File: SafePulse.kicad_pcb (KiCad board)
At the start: 4 copper layers, 40.6 x 20.8 mm, 88 parts, among them IC1 S-35770E01I-K8T2U, J1 Conn_01x03_Male, J2 4208, Q1 FQT7N10L, Q2 BC846A, Q3 MMBT3906, Q4 MMBT3906, U1 TS4061AICT-1.25, U2 74HC14, U3 TLV27L1DBVT, U33 MAX9910EXK+T, U4 CD14538BM

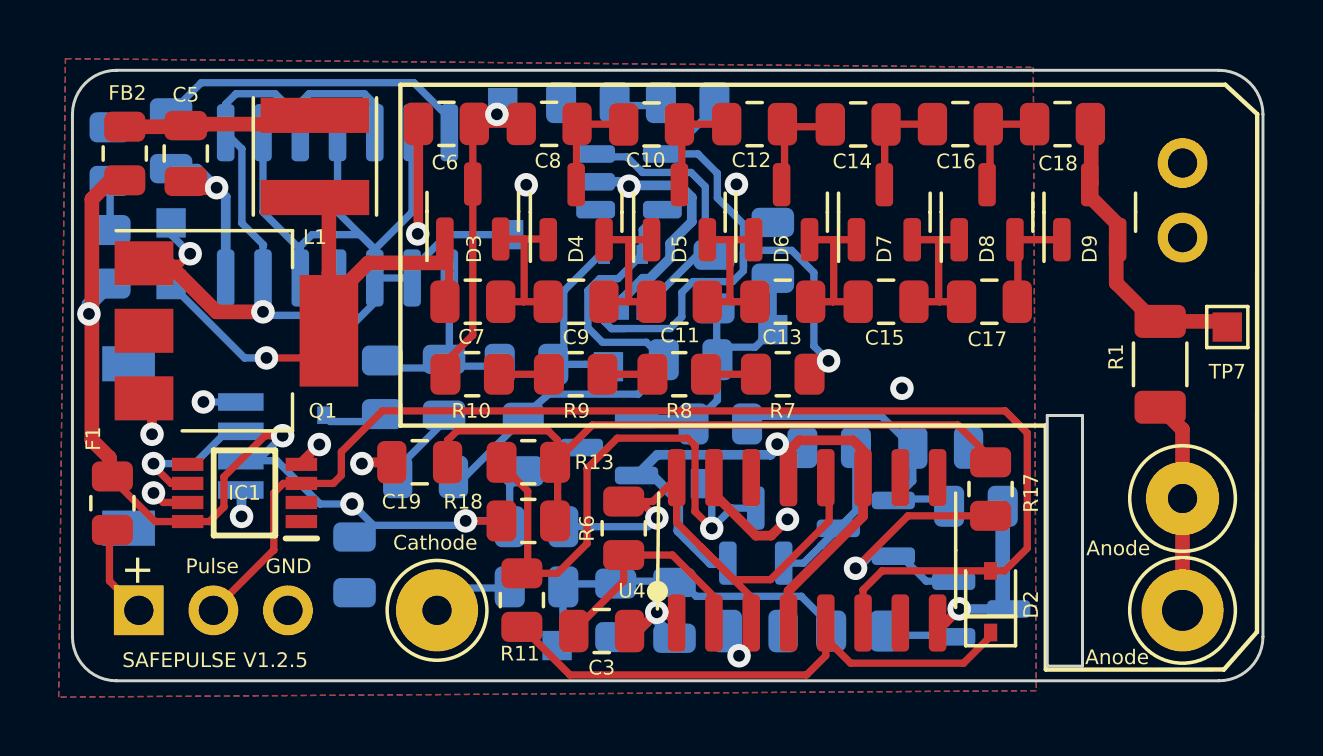
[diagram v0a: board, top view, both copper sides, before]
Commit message: Updated V1.2.4 board with new JCLPCB number
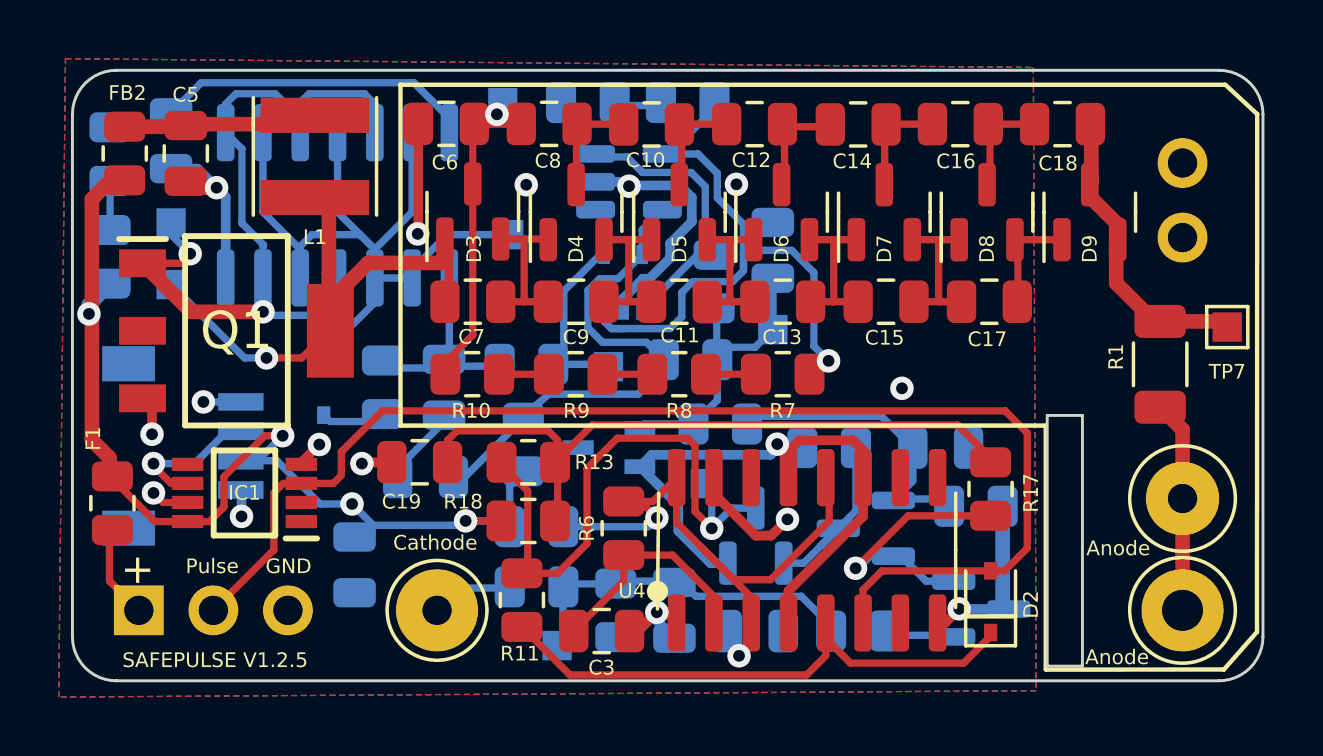
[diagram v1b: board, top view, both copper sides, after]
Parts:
- Q1: footprint Package_TO_SOT_SMD:SOT-223-3_TabPin4 -> Library:SOT230P700X180-4N
- U1: footprint Package_TO_SOT_SMD:SOT-23 -> Library:SOT65P210X110-3N
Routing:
- net GND: track 64.3 -> 63.6 mm
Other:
- copper layers 4 -> 13

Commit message: V1.2.5 boards
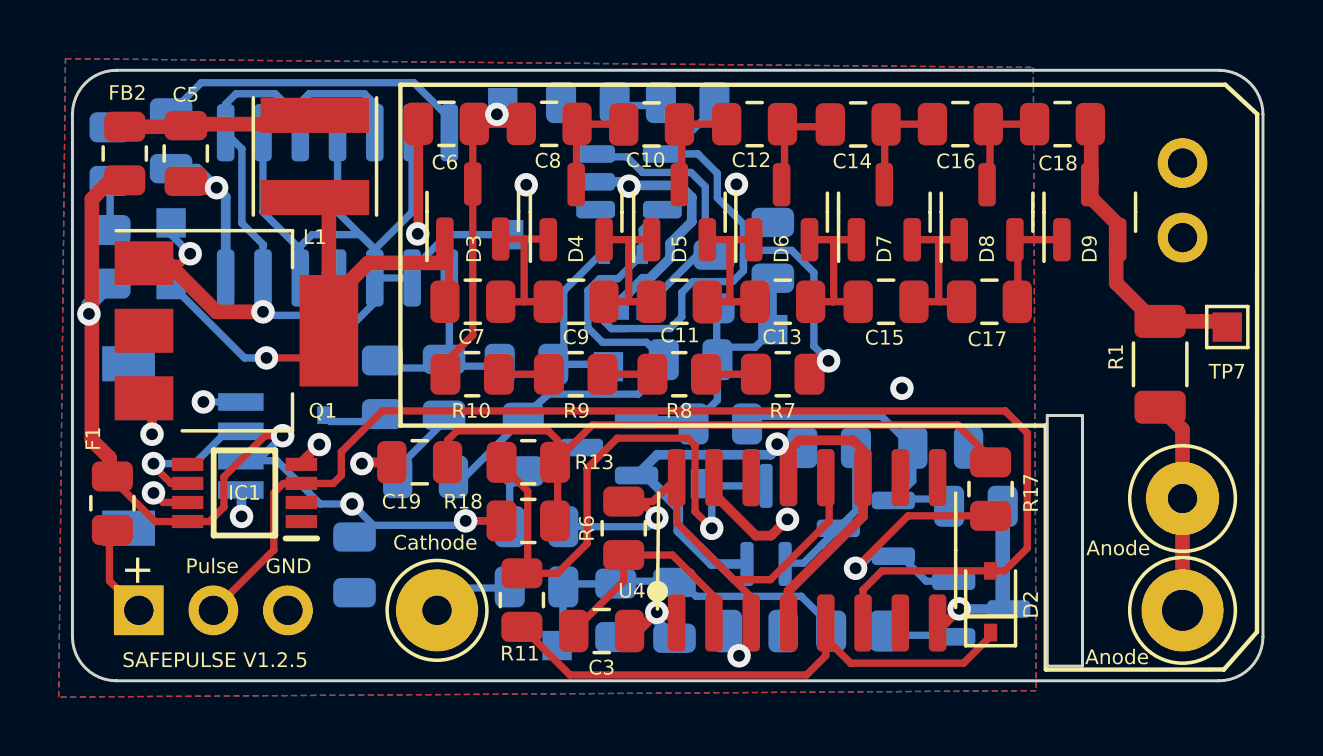
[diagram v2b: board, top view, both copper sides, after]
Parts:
- Q1: footprint Library:SOT230P700X180-4N -> Package_TO_SOT_SMD:SOT-223-3_TabPin4
- Q2: footprint Package_TO_SOT_SMD:SOT-23 -> Package_TO_SOT_SMD:SOT-323_SC-70_Handsoldering
- U1: footprint Library:SOT65P210X110-3N -> Package_TO_SOT_SMD:SOT-23
- moved Q2 0.51 mm to (149.9, 72.7)
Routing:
- net GND: track 63.6 -> 64.9 mm
